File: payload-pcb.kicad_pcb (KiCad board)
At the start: 4 copper layers, 127 x 76.2 mm, 112 parts, among them J1 POWER_IN, J10 GPIO0, J12 I2C, J13 GPIO1, J14 CAN, J15 CAN, J16 SCOOP1, J17 SCOOP2, J18 ACTUATOR, J19 DRILL, J2 POWER_OUT, J20 SERVO5, J21 SERVO6, J22 SERVO7, J23 SERVO8, J5 MOIST, J6 TEMP, J7 POT3, J9 RELAYS, Q1 SUD50P10-43L-GE3, Q2 SUD50P10-43L-GE3, Q3 SUD50P10-43L-GE3, Q4 DMG2305UX, Q5 Q_NMOS, Q6 Q_NMOS, Q7 Q_NMOS, Q8 Q_NMOS, U12 +3V3@2A, U14 Pico, U15 74HCT244, U22 MCP2562, U23 MCP2515, U8 PCA9555PWR, U9 +5V@2A, Y1 8MHz

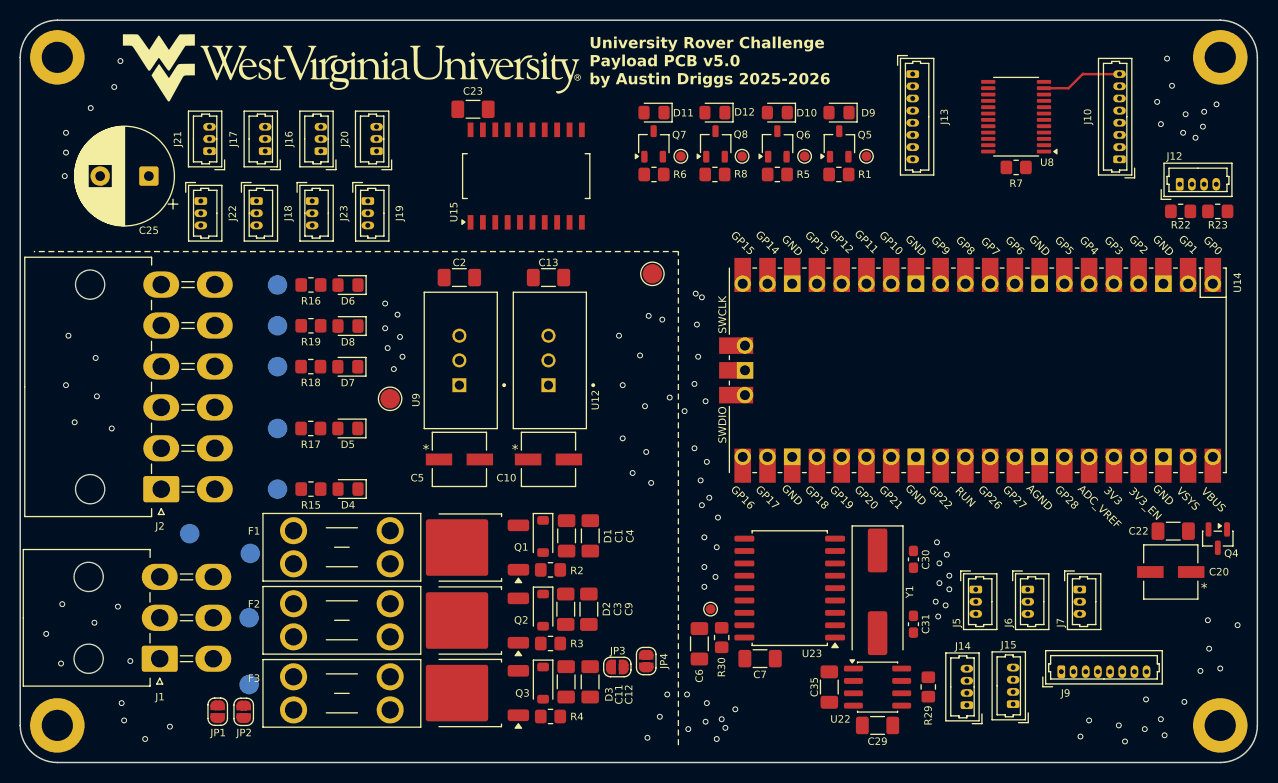
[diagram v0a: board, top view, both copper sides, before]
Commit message: major rework again after the meeting
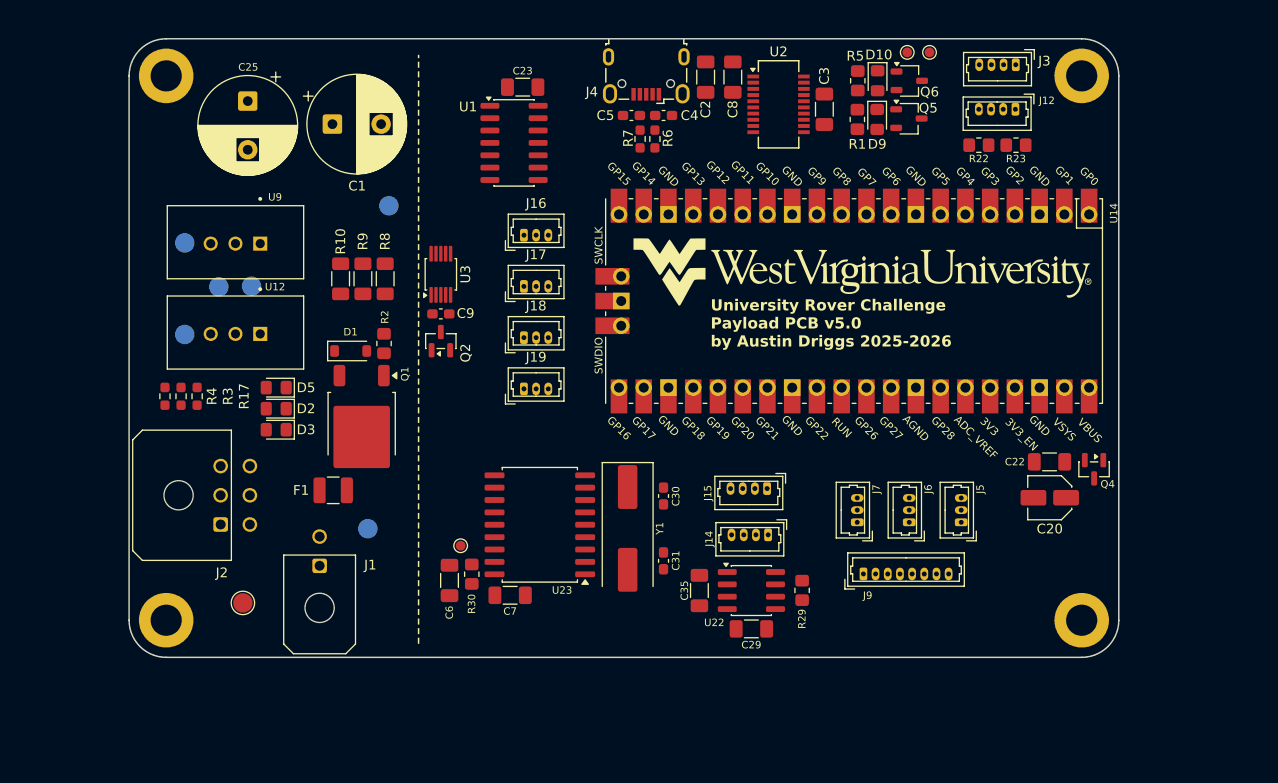
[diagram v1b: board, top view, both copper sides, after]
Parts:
- removed C10: 22 uF, Payload_PCB_v3.1:UCM1H220MCL1GS
- removed C11, C12, C13: 0.1 uF, Capacitor_SMD:C_1206_3216Metric_Pad1.33x1.80mm_HandSolder
- removed D11: LED4, LED_SMD:LED_0805_2012Metric_Pad1.15x1.40mm_HandSolder
- removed D12: LED3, LED_SMD:LED_0805_2012Metric_Pad1.15x1.40mm_HandSolder
- removed D4: +40V, LED_SMD:LED_0805_2012Metric_Pad1.15x1.40mm_HandSolder
- removed D6: VDC, LED_SMD:LED_0805_2012Metric_Pad1.15x1.40mm_HandSolder
- removed D7: +5V, LED_SMD:LED_0805_2012Metric_Pad1.15x1.40mm_HandSolder
- removed D8: +3V3, LED_SMD:LED_0805_2012Metric_Pad1.15x1.40mm_HandSolder
- removed F2, F3: Fuse, Fuse:Fuseholder_Blade_Mini_Keystone_3568
- removed J10: GPIO0, Connector_Molex:Molex_PicoBlade_53047-0810_1x08_P1.25mm_Vertical
- removed J13: GPIO1, Connector_Molex:Molex_PicoBlade_53047-0810_1x08_P1.25mm_Vertical
- removed J20: SERVO5, Connector_Molex:Molex_PicoBlade_53047-0310_1x03_P1.25mm_Vertical
- removed J21: SERVO6, Connector_Molex:Molex_PicoBlade_53047-0310_1x03_P1.25mm_Vertical
- removed J22: SERVO7, Connector_Molex:Molex_PicoBlade_53047-0310_1x03_P1.25mm_Vertical
- removed J23: SERVO8, Connector_Molex:Molex_PicoBlade_53047-0310_1x03_P1.25mm_Vertical
- removed JP1, JP2, JP3, JP4: SolderJumper_2_Open, Jumper:SolderJumper-2_P1.3mm_Open_RoundedPad1.0x1.5mm
- removed Q3: SUD50P10-43L-GE3, Package_TO_SOT_SMD:TO-252-2
- removed Q7, Q8: Q_NMOS, Package_TO_SOT_SMD:TSOT-23
- removed R15: 1k, Resistor_SMD:R_0805_2012Metric_Pad1.20x1.40mm_HandSolder
- removed R16, R18: 150, Resistor_SMD:R_0805_2012Metric_Pad1.20x1.40mm_HandSolder
- removed R19: 62, Resistor_SMD:R_0805_2012Metric_Pad1.20x1.40mm_HandSolder
- removed TP14: LED4, TestPoint:TestPoint_Pad_D1.0mm
- removed TP16: LED3, TestPoint:TestPoint_Pad_D1.0mm
- removed TP2: +BATT_IN, TestPoint:TestPoint_Pad_D2.0mm
- removed TP3: +VDC_IN, TestPoint:TestPoint_Pad_D2.0mm
- removed TP4, TP6: +12V_IN, TestPoint:TestPoint_Pad_D2.0mm
- removed U15: 74HCT244, Package_SO:SO-20_12.8x7.5mm_P1.27mm
- removed U8: PCA9555PWR, Package_SO:TSSOP-24_4.4x7.8mm_P0.65mm
- added C8: 0.1 uF, Capacitor_SMD:C_1206_3216Metric_Pad1.33x1.80mm_HandSolder, F.Cu at (162.1, 69.3)
- added J3: UART, Connector_Molex:Molex_PicoBlade_53047-0410_1x04_P1.25mm_Vertical, F.Cu at (191.1, 68.1)
- added J4: USB, Connector_USB:USB_Micro-B_Wuerth_629105150521, F.Cu at (153.2, 69.2)
- added R10: 45m, Resistor_SMD:R_1206_3216Metric_Pad1.30x1.75mm_HandSolder, F.Cu at (121.8, 90.0)
- added R9: 45m, Resistor_SMD:R_1206_3216Metric_Pad1.30x1.75mm_HandSolder, F.Cu at (124.1, 90.0)
- added U1: SN74AHCT126DR, Package_SO:SOIC-14_3.9x8.7mm_P1.27mm, F.Cu at (139.6, 76.1)
- added U2: FT230XS, Package_SO:SSOP-20_3.9x8.7mm_P0.635mm, F.Cu at (166.8, 72.1)
- added U3: LTC2990, Package_SO:MSOP-10_3x3mm_P0.5mm, F.Cu at (132.1, 89.6)
- C1: value 0.1 uF -> 22 uF; footprint Capacitor_SMD:C_1206_3216Metric_Pad1.33x1.80mm_HandSolder -> Capacitor_THT:CP_Radial_D10.0mm_P5.00mm
- C20: footprint Payload_PCB_v3.1:UCM1H220MCL1GS -> Capacitor_SMD:C_Elec_4x5.4
- C4: value 0.1 uF -> 47p; footprint Capacitor_SMD:C_1206_3216Metric_Pad1.33x1.80mm_HandSolder -> Capacitor_SMD:C_0603_1608Metric_Pad1.08x0.95mm_HandSolder
- C5: value 22 uF -> 47p; footprint Payload_PCB_v3.1:UCM1H220MCL1GS -> Capacitor_SMD:C_0603_1608Metric_Pad1.08x0.95mm_HandSolder
- C9: value 0.1 uF -> 470p; footprint Capacitor_SMD:C_1206_3216Metric_Pad1.33x1.80mm_HandSolder -> Capacitor_SMD:C_0603_1608Metric_Pad1.08x0.95mm_HandSolder
- D10: value LED2 -> BAD
- D2, D3: value BZT52C10-TP -> +12V; footprint Diode_SMD:D_SOD-123 -> LED_SMD:LED_0805_2012Metric_Pad1.15x1.40mm_HandSolder
- D9: value LED1 -> GOOD
- F1: footprint Fuse:Fuseholder_Blade_Mini_Keystone_3568 -> Fuse:Fuse_1210_3225Metric
- J1: footprint Connector_Molex:Molex_Mini-Fit_Jr_5569-06A2_2x03_P4.20mm_Horizontal -> Connector_Molex:Molex_Micro-Fit_3.0_43045-0200_2x01_P3.00mm_Horizontal
- J16: value SCOOP1 -> SCOOP
- J17: value SCOOP2 -> MANIPULATOR
- J18: value ACTUATOR -> SERVO3
- J19: value DRILL -> SERVO4
- J2: footprint Connector_Molex:Molex_Mini-Fit_Jr_5569-12A2_2x06_P4.20mm_Horizontal -> Connector_Molex:Molex_Micro-Fit_3.0_43045-0600_2x03_P3.00mm_Horizontal
- J7: value POT3 -> MANIPULATOR
- J9: value RELAYS -> GPIO
- Q2: value SUD50P10-43L-GE3 -> MMBT3904; footprint Package_TO_SOT_SMD:TO-252-2 -> Package_TO_SOT_SMD:SOT-23
- R17: footprint Resistor_SMD:R_0805_2012Metric_Pad1.20x1.40mm_HandSolder -> Resistor_SMD:R_0603_1608Metric_Pad0.98x0.95mm_HandSolder
- R3, R4: value 100k -> 511; footprint Resistor_SMD:R_0805_2012Metric_Pad1.20x1.40mm_HandSolder -> Resistor_SMD:R_0603_1608Metric_Pad0.98x0.95mm_HandSolder
- R6: value 511 -> 27; footprint Resistor_SMD:R_0805_2012Metric_Pad1.20x1.40mm_HandSolder -> Resistor_SMD:R_0603_1608Metric_Pad0.98x0.95mm_HandSolder
- R7: value 10k -> 27; footprint Resistor_SMD:R_0805_2012Metric_Pad1.20x1.40mm_HandSolder -> Resistor_SMD:R_0603_1608Metric_Pad0.98x0.95mm_HandSolder
- R8: value 511 -> 45m; footprint Resistor_SMD:R_0805_2012Metric_Pad1.20x1.40mm_HandSolder -> Resistor_SMD:R_1206_3216Metric_Pad1.30x1.75mm_HandSolder
- TP11: moved to B.Cu
- U14: value Pico -> PI_PICO
- moved C3 57.8 mm to (171.4, 72.6), turned to -90 degrees
- moved G*** 56.5 mm to (175.4, 89.4)
- moved TP10 53.9 mm to (111.8, 123.3), turned to 90 degrees
- moved R4 51.4 mm to (103.8, 102.1), turned to -90 degrees
- moved C1 48.6 mm to (120.9, 74.2), turned to 0 degrees
- moved R3 45.6 mm to (105.4, 102.1), turned to -90 degrees
- moved C4 43.8 mm to (154.9, 73.3), turned to 180 degrees
- moved C5 39.5 mm to (151.6, 73.3)
- moved TP9 39.4 mm to (126.7, 82.5), turned to -90 degrees
- moved R7 38.7 mm to (152.5, 75.7), turned to -90 degrees
- moved D3 37.8 mm to (115.2, 105.5), turned to 180 degrees
- moved R8 35.5 mm to (126.4, 90.0), turned to 90 degrees
- moved D2 34.3 mm to (115.2, 103.4), turned to 180 degrees
- moved C9 33.9 mm to (132.1, 93.6), turned to 180 degrees
- moved J15 33.6 mm to (165.6, 111.6), turned to 180 degrees
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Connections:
- net ANALOG_POT3 renamed ANALOG_MANIPULATOR
- net DIGITAL_GP14 renamed DIGITAL_LIMIT_SW1
- net DIGITAL_GP15 renamed DIGITAL_LIMIT_SW2
- net DIGITAL_GP21 renamed DIGITAL_RELAY1
- net DIGITAL_GP22 renamed DIGITAL_RELAY2
- net LED1 renamed /Pi Pico/LED_GOOD
- net LED2 renamed /Pi Pico/LED_BAD
- C1 pad 1: GND -> +12V
- C1 pad 2: +12V -> GND
- C2 pad 2: +3.3V -> +5V
- C25 pad 1: VDC -> +5V
- C3 pad 2: +BATT -> +5V
- C4 pad 2: +12V -> /USB/USB-
- C5 pad 1: +12V -> GND
- C5 pad 2: GND -> /USB/USB+
- C9 pad 1: GND -> Net-(Q2-E)
- C9 pad 2: +BATT -> Net-(Q2-B)
- D1 pad 1: +12V -> /Power/+12V_PROTECTED
- D10 pad 1: GND -> Net-(D10-K)
- D2 pad 1: +BATT -> GND
- D3 pad 1: Net-(D3-K) -> GND
- D9 pad 1: GND -> Net-(D9-K)
- J1 pad 2: GND -> /Power/+12V_IN
- J12 pad 2: I2C0_SCL -> I2C0_SDA
- J12 pad 3: I2C0_SDA -> I2C0_SCL
- J16 pad 1: VDC -> +5V
- J17 pad 1: VDC -> +5V
- J18 pad 1: VDC -> +5V
- J19 pad 1: VDC -> +5V
- J2 pad 4: GND -> +12V
- J2 pad 5: GND -> +5V
- J2 pad 6: GND -> +3.3V
- Q1 pad 3: +12V -> /Power/+12V_PROTECTED
- Q2 pad 1: Net-(D2-A) -> Net-(Q2-B)
- Q2 pad 2: Net-(Q2-D) -> Net-(Q2-E)
- Q2 pad 3: +BATT -> Net-(Q2-B)
- Q4 pad 3: +3.3V -> +5V
- Q5 pad 1: Net-(Q5-D) -> Net-(D9-K)
- Q5 pad 3: Net-(D9-A) -> GND
- Q6 pad 1: Net-(Q6-D) -> Net-(D10-K)
- Q6 pad 3: Net-(D10-A) -> GND
- R1 pad 1: Net-(Q5-D) -> Net-(D9-A)
- R3 pad 2: GND -> +5V
- R4 pad 2: GND -> +3.3V
- R5 pad 1: Net-(Q6-D) -> Net-(D10-A)
- R6 pad 1: Net-(Q7-D) -> /USB/USB-
- R6 pad 2: +3.3V -> Net-(U2-USBDM)
- R7 pad 1: Net-(U8-~{INT}) -> /USB/USB+
- R7 pad 2: +3.3V -> Net-(U2-USBDP)
- R8 pad 1: Net-(Q8-D) -> /Power/+12V_PROTECTED
- R8 pad 2: +3.3V -> +12V
- U14 pad 10: SERVO6_PICO -> unconnected-(U14-GPIO7-Pad10)
- U14 pad 11: SERVO7_PICO -> /Pi Pico/UART1_TX
- U14 pad 12: SERVO8_PICO -> /Pi Pico/UART1_RX
- U14 pad 16: LED3 -> UART0_TX
- U14 pad 17: LED4 -> UART0_RX
- U14 pad 9: SERVO5_PICO -> unconnected-(U14-GPIO6-Pad9)
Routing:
- net Net-(J10-Pin_8): track 8.38 -> 0.00 mm
- net (no net): vias 102 -> 0
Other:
- board size 127 x 76.2 mm -> 101.6 x 63.5 mm
